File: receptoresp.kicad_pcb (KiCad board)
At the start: 2 copper layers, 48 x 59 mm, 7 parts

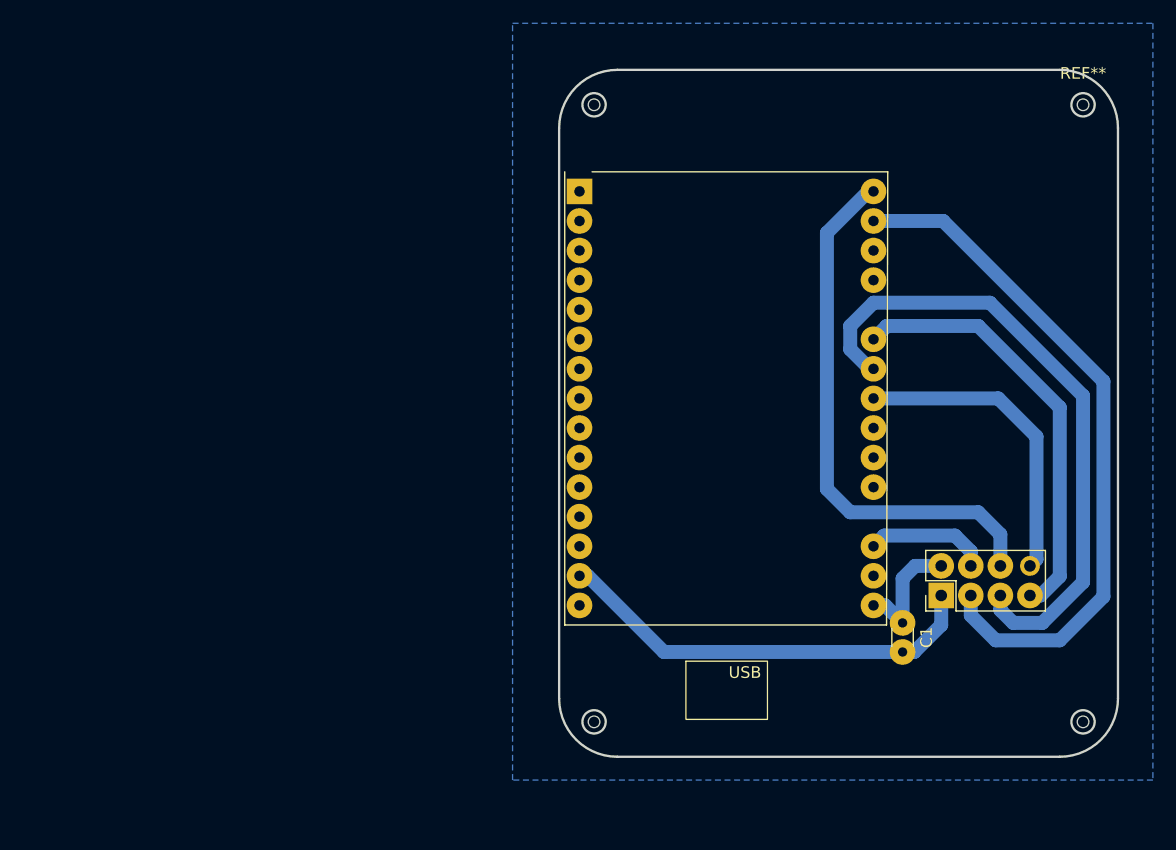
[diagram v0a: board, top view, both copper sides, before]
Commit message: pcb pi pico
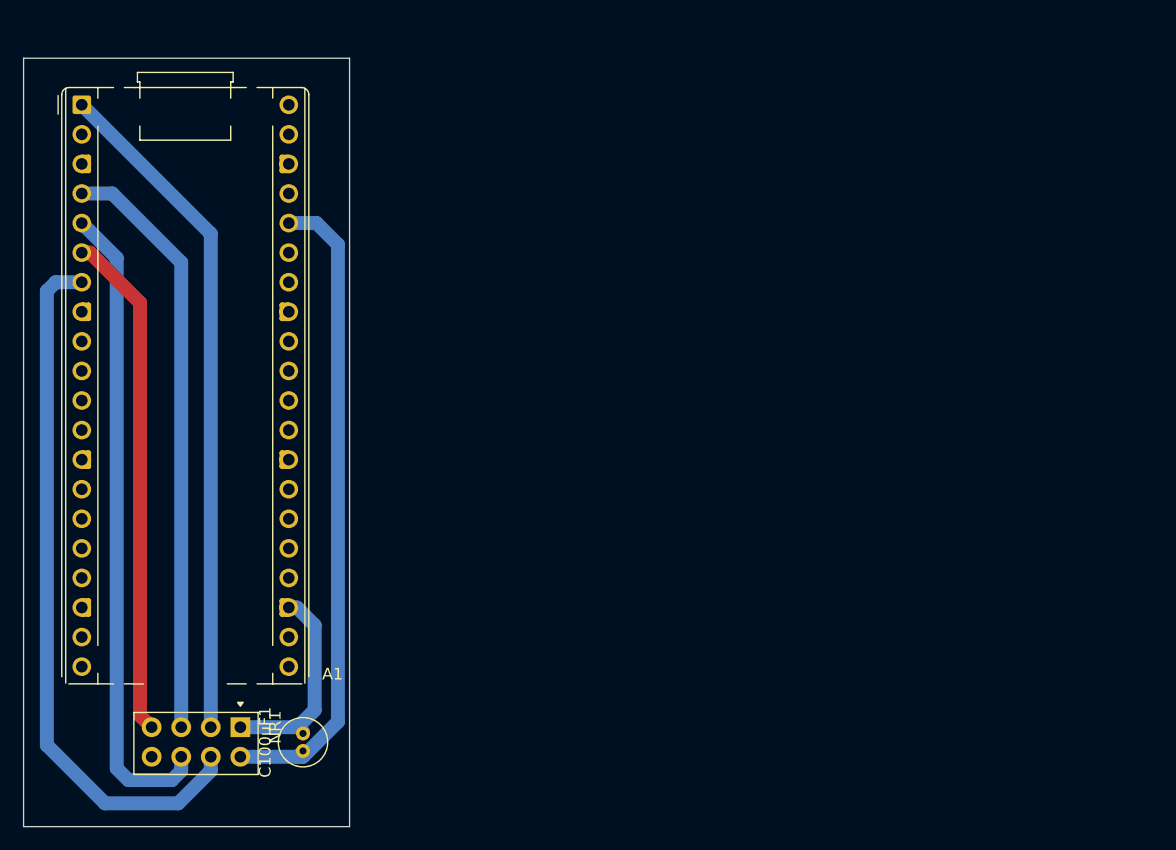
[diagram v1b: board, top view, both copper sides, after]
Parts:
- removed ? (x3): , 
- removed C1: C_Polarized, Capacitor_THT:C_Disc_D3.0mm_W1.6mm_P2.50mm
- removed E1: ESP-WROOM-32, ESPF:ESP-WROOM-32
- removed REF**: MountingHole_2.2mm_M2_ISO7380, MountingHole:MountingHole_2.2mm_M2_ISO7380
- added A1: RaspberryPi_Pico, Module:RaspberryPi_Pico_Common_THT, F.Cu at (83.0, 57.0)
- added C100uF1: C_Polarized, Capacitor_THT:C_Radial_D4.0mm_H5.0mm_P1.50mm, F.Cu at (102.0, 112.5)
- NR1: footprint nrf:NRF24L01 -> RF_Module:nRF24L01_Breakout
- moved NR1 77.5 mm to (96.6, 110.5), turned to -90 degrees
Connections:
- NR1 pad 8: Net-(E1-D5) -> unconnected-(NR1-IRQ-Pad8)
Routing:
- net Net-(A1-GPIO5): track 10.5 -> 60.8 mm
- net Net-(A1-3V3): track 10.7 -> 56.2 mm
- net Net-(E1-D5): track 26.7 -> 0.00 mm
- net Net-(NR1-GND): track 37.3 -> 17.7 mm
- net Net-(A1-GPIO3): track 46.7 -> 55.6 mm
- net Net-(A1-GPIO4): track 37.1 -> 43.7 mm
- net Net-(A1-GPIO2): track 55.1 -> 50.9 mm
- net Net-(A1-GPIO0): track 59.5 -> 58.0 mm
- removed copper zone on B.Cu, net (none)
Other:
- board size 48 x 59 mm -> 28 x 66 mm
